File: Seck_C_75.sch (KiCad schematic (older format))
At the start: 122 parts, among them SW1 RESET, U1 ATmega32U4-AU, Y1 16MHz

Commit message: Layout
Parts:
- removed D1, D10, D11, D12, D13, D14, D15, D16, D17, D18, D19, D2, D20, D21, D22, D23, D24, D25, D26, D27, D28, D29, D3, D30, D31, D32, D4, D5, D6, D7, D8, D9: BAV70, Custom_Footprints:SOT-23_Annotated, symbol Diode:BAV70
- removed K_0: KC_ESC, MX_Only:MXOnly-1U-NoLED, symbol Switch:SW_Push
- removed K_013A1: KC_BSPC, MX_Only:MXOnly-1U-NoLED, symbol Switch:SW_Push
- removed K_100: KC_TAB, MX_Only:MXOnly-1.5U-NoLED, symbol Switch:SW_Push
- removed K_101: KC_Q, MX_Only:MXOnly-1U-NoLED, symbol Switch:SW_Push
- removed K_102: KC_W, MX_Only:MXOnly-1U-NoLED, symbol Switch:SW_Push
- removed K_103: KC_E, MX_Only:MXOnly-1U-NoLED, symbol Switch:SW_Push
- removed K_104: KC_R, MX_Only:MXOnly-1U-NoLED, symbol Switch:SW_Push
- removed K_105: KC_T, MX_Only:MXOnly-1U-NoLED, symbol Switch:SW_Push
- removed K_106: KC_Y, MX_Only:MXOnly-1U-NoLED, symbol Switch:SW_Push
- removed K_107: KC_U, MX_Only:MXOnly-1U-NoLED, symbol Switch:SW_Push
- removed K_108: KC_I, MX_Only:MXOnly-1U-NoLED, symbol Switch:SW_Push
- removed K_109: KC_O, MX_Only:MXOnly-1U-NoLED, symbol Switch:SW_Push
- removed K_110: KC_P, MX_Only:MXOnly-1U-NoLED, symbol Switch:SW_Push
- removed K_111: KC_LBRC, MX_Only:MXOnly-1U-NoLED, symbol Switch:SW_Push
- removed K_112: KC_RBRC, MX_Only:MXOnly-1U-NoLED, symbol Switch:SW_Push
- removed K_113: KC_BSLS, MX_Only:MXOnly-1.5U-NoLED, symbol Switch:SW_Push
- removed K_200: KC_CAPS, MX_Only:MXOnly-1.75U-NoLED, symbol Switch:SW_Push
- removed K_200A1: KC_CAPS, MX_Only:MXOnly-1.25U-NoLED, symbol Switch:SW_Push
- removed K_201: KC_A, MX_Only:MXOnly-1U-NoLED, symbol Switch:SW_Push
- removed K_202: KC_S, MX_Only:MXOnly-1U-NoLED, symbol Switch:SW_Push
- removed K_203: KC_D, MX_Only:MXOnly-1U-NoLED, symbol Switch:SW_Push
- removed K_204: KC_F, MX_Only:MXOnly-1U-NoLED, symbol Switch:SW_Push
- removed K_205: KC_G, MX_Only:MXOnly-1U-NoLED, symbol Switch:SW_Push
- removed K_206: KC_H, MX_Only:MXOnly-1U-NoLED, symbol Switch:SW_Push
- removed K_207: KC_J, MX_Only:MXOnly-1U-NoLED, symbol Switch:SW_Push
- removed K_208: KC_K, MX_Only:MXOnly-1U-NoLED, symbol Switch:SW_Push
- removed K_209: KC_L, MX_Only:MXOnly-1U-NoLED, symbol Switch:SW_Push
- removed K_210: KC_SCLN, MX_Only:MXOnly-1U-NoLED, symbol Switch:SW_Push
- removed K_211: KC_QUOT, MX_Only:MXOnly-1U-NoLED, symbol Switch:SW_Push
- removed K_212: KC_ENT, MX_Only:MXOnly-2.25U-NoLED, symbol Switch:SW_Push
- removed K_213: KC_DEL, MX_Only:MXOnly-1U-NoLED, symbol Switch:SW_Push
- removed K_300: KC_LSFT, MX_Only:MXOnly-2.25U-NoLED, symbol Switch:SW_Push
- removed K_301: KC_Z, MX_Only:MXOnly-1U-NoLED, symbol Switch:SW_Push
- removed K_302: KC_X, MX_Only:MXOnly-1U-NoLED, symbol Switch:SW_Push
- removed K_303: KC_C, MX_Only:MXOnly-1U-NoLED, symbol Switch:SW_Push
- removed K_304: KC_V, MX_Only:MXOnly-1U-NoLED, symbol Switch:SW_Push
- removed K_305: KC_B, MX_Only:MXOnly-1U-NoLED, symbol Switch:SW_Push
- removed K_306: KC_N, MX_Only:MXOnly-1U-NoLED, symbol Switch:SW_Push
- removed K_307: KC_M, MX_Only:MXOnly-1U-NoLED, symbol Switch:SW_Push
- removed K_308: KC_COMM, MX_Only:MXOnly-1U-NoLED, symbol Switch:SW_Push
- removed K_309: KC_DOT, MX_Only:MXOnly-1U-NoLED, symbol Switch:SW_Push
- removed K_310: KC_SLSH, MX_Only:MXOnly-1U-NoLED, symbol Switch:SW_Push
- removed K_311: KC_RSFT, MX_Only:MXOnly-2.75U-NoLED, symbol Switch:SW_Push
- removed K_311A1: KC_RSFT, MX_Only:MXOnly-1.75U-NoLED, symbol Switch:SW_Push
- removed K_312, K_410A1: KC_MO(1), MX_Only:MXOnly-1U-NoLED, symbol Switch:SW_Push
- removed K_400: KC_LCTL, MX_Only:MXOnly-1.25U-NoLED, symbol Switch:SW_Push
- removed K_400A1: KC_LCTL, MX_Only:MXOnly-1.5U-NoLED, symbol Switch:SW_Push
- removed K_401: KC_LGUI, MX_Only:MXOnly-1.25U-NoLED, symbol Switch:SW_Push
- removed K_401A1: KC_LGUI, MX_Only:MXOnly-1U-NoLED, symbol Switch:SW_Push
- removed K_402: KC_LALT, MX_Only:MXOnly-1.25U-NoLED, symbol Switch:SW_Push
- removed K_402A1: KC_LALT, MX_Only:MXOnly-1.5U-NoLED, symbol Switch:SW_Push
- removed K_406: KC_SPC, MX_Only:MXOnly-6.25U-ReversedStabilizers-NoLED, symbol Switch:SW_Push
- removed K_406A1: KC_SPC, MX_Only:MXOnly-7U-ReversedStabilizers-NoLED, symbol Switch:SW_Push
- removed K_408: KC_RALT, MX_Only:MXOnly-1.25U-NoLED, symbol Switch:SW_Push
- removed K_409: KC_RGUI, MX_Only:MXOnly-1.25U-NoLED, symbol Switch:SW_Push
- removed K_409A1: KC_RALT, MX_Only:MXOnly-1.5U-NoLED, symbol Switch:SW_Push
- removed K_410: KC_MO(1), MX_Only:MXOnly-1.25U-NoLED, symbol Switch:SW_Push
- removed K_411: KC_RCTL, MX_Only:MXOnly-1.25U-NoLED, symbol Switch:SW_Push
- removed K_411A1: KC_RCTL, MX_Only:MXOnly-1.5U-NoLED, symbol Switch:SW_Push
- added D1, D10, D11, D12, D13, D14, D15, D16, D17, D18, D19, D2, D20, D21, D22, D23, D24, D25, D26, D27, D28, D29, D3, D30, D31, D32, D33, D34, D35, D36, D37, D38, D39, D4, D40, D41, D42, D43, D44, D45, D46, D47, D48, D49, D5, D50, D51, D52, D53, D54, D55, D56, D57, D58, D59, D6, D60, D61, D62, D63, D64, D65, D66, D67, D68, D69, D7, D70, D71, D72, D73, D74, D75, D76, D77, D78, D79, D8, D80, D81, D82, D9: D_Small, Custom_Footprints:D_SOD-123_Annotated, symbol Device:D_Small
- added J1: OLED, Custom_Footprints:SSD1306_OLED, symbol Connector:Conn_01x04_Female
- added K_113A1: KC_BSPC, MX_Only:MXOnly-1U-NoLED, symbol Switch:SW_Push
- added K_14: KC_GRV, MX_Only:MXOnly-1U-NoLED, symbol Switch:SW_Push
- added K_15: KC_1, MX_Only:MXOnly-1U-NoLED, symbol Switch:SW_Push
- added K_16: KC_2, MX_Only:MXOnly-1U-NoLED, symbol Switch:SW_Push
- added K_17: KC_3, MX_Only:MXOnly-1U-NoLED, symbol Switch:SW_Push
- added K_18: KC_4, MX_Only:MXOnly-1U-NoLED, symbol Switch:SW_Push
- added K_19: KC_5, MX_Only:MXOnly-1U-NoLED, symbol Switch:SW_Push
- added K_20: KC_6, MX_Only:MXOnly-1U-NoLED, symbol Switch:SW_Push
- added K_21: KC_7, MX_Only:MXOnly-1U-NoLED, symbol Switch:SW_Push
- added K_22: KC_8, MX_Only:MXOnly-1U-NoLED, symbol Switch:SW_Push
- added K_23: KC_9, MX_Only:MXOnly-1U-NoLED, symbol Switch:SW_Push
- added K_24: KC_0, MX_Only:MXOnly-1U-NoLED, symbol Switch:SW_Push
- added K_25: KC_MINS, MX_Only:MXOnly-1U-NoLED, symbol Switch:SW_Push
- added K_26: KC_EQL, MX_Only:MXOnly-1U-NoLED, symbol Switch:SW_Push
- added K_27: KC_BSPC, MX_Only:MXOnly-2U-NoLED, symbol Switch:SW_Push
- added K_28: KC_DEL, MX_Only:MXOnly-1U-NoLED, symbol Switch:SW_Push
- added K_29: KC_TAB, MX_Only:MXOnly-1.5U-NoLED, symbol Switch:SW_Push
- added K_30: KC_Q, MX_Only:MXOnly-1U-NoLED, symbol Switch:SW_Push
- added K_300A1: KC_CAPS, MX_Only:MXOnly-1.25U-NoLED, symbol Switch:SW_Push
- added K_31: KC_W, MX_Only:MXOnly-1U-NoLED, symbol Switch:SW_Push
- added K_32: KC_E, MX_Only:MXOnly-1U-NoLED, symbol Switch:SW_Push
- added K_33: KC_R, MX_Only:MXOnly-1U-NoLED, symbol Switch:SW_Push
- added K_34: KC_T, MX_Only:MXOnly-1U-NoLED, symbol Switch:SW_Push
- added K_35: KC_Y, MX_Only:MXOnly-1U-NoLED, symbol Switch:SW_Push
- added K_36: KC_U, MX_Only:MXOnly-1U-NoLED, symbol Switch:SW_Push
- added K_37: KC_I, MX_Only:MXOnly-1U-NoLED, symbol Switch:SW_Push
- added K_38: KC_O, MX_Only:MXOnly-1U-NoLED, symbol Switch:SW_Push
- added K_39: KC_P, MX_Only:MXOnly-1U-NoLED, symbol Switch:SW_Push
- added K_40: KC_LBRC, MX_Only:MXOnly-1U-NoLED, symbol Switch:SW_Push
- added K_41: KC_RBRC, MX_Only:MXOnly-1U-NoLED, symbol Switch:SW_Push
- added K_42: KC_BSLS, MX_Only:MXOnly-1.5U-NoLED, symbol Switch:SW_Push
- added K_43: KC_INS, MX_Only:MXOnly-1U-NoLED, symbol Switch:SW_Push
- added K_44: KC_CAPS, MX_Only:MXOnly-1.75U-NoLED, symbol Switch:SW_Push
- added K_45: KC_A, MX_Only:MXOnly-1U-NoLED, symbol Switch:SW_Push
- added K_46: KC_S, MX_Only:MXOnly-1U-NoLED, symbol Switch:SW_Push
- added K_47: KC_D, MX_Only:MXOnly-1U-NoLED, symbol Switch:SW_Push
- added K_48: KC_F, MX_Only:MXOnly-1U-NoLED, symbol Switch:SW_Push
- added K_49: KC_G, MX_Only:MXOnly-1U-NoLED, symbol Switch:SW_Push
- added K_50: KC_H, MX_Only:MXOnly-1U-NoLED, symbol Switch:SW_Push
- added K_508A1: KC_, MX_Only:MXOnly-1.5U-NoLED, symbol Switch:SW_Push
- added K_51: KC_J, MX_Only:MXOnly-1U-NoLED, symbol Switch:SW_Push
- added K_510A1: KC_RCTL, MX_Only:MXOnly-1.5U-NoLED, symbol Switch:SW_Push
- added K_52: KC_K, MX_Only:MXOnly-1U-NoLED, symbol Switch:SW_Push
- added K_53: KC_L, MX_Only:MXOnly-1U-NoLED, symbol Switch:SW_Push
- added K_54: KC_SCLN, MX_Only:MXOnly-1U-NoLED, symbol Switch:SW_Push
- added K_55: KC_QUOT, MX_Only:MXOnly-1U-NoLED, symbol Switch:SW_Push
- added K_56: KC_ENT, MX_Only:MXOnly-2.25U-NoLED, symbol Switch:SW_Push
- added K_57: KC_BSLS, MX_Only:MXOnly-1U-NoLED, symbol Switch:SW_Push
- added K_58: KC_HOME, MX_Only:MXOnly-1U-NoLED, symbol Switch:SW_Push
- added K_59: KC_LSFT, MX_Only:MXOnly-2.25U-NoLED, symbol Switch:SW_Push
- added K_60: KC_Z, MX_Only:MXOnly-1U-NoLED, symbol Switch:SW_Push
- added K_61: KC_X, MX_Only:MXOnly-1U-NoLED, symbol Switch:SW_Push
- added K_62: KC_C, MX_Only:MXOnly-1U-NoLED, symbol Switch:SW_Push
- added K_63: KC_V, MX_Only:MXOnly-1U-NoLED, symbol Switch:SW_Push
- added K_64: KC_B, MX_Only:MXOnly-1U-NoLED, symbol Switch:SW_Push
- added K_65: KC_N, MX_Only:MXOnly-1U-NoLED, symbol Switch:SW_Push
- added K_66: KC_M, MX_Only:MXOnly-1U-NoLED, symbol Switch:SW_Push
- added K_67: KC_COMM, MX_Only:MXOnly-1U-NoLED, symbol Switch:SW_Push
- added K_68: KC_DOT, MX_Only:MXOnly-1U-NoLED, symbol Switch:SW_Push
- added K_69: KC_SLSH, MX_Only:MXOnly-1U-NoLED, symbol Switch:SW_Push
- added K_70: KC_RSFT, MX_Only:MXOnly-1.75U-NoLED, symbol Switch:SW_Push
- added K_71: KC_UP, MX_Only:MXOnly-1U-NoLED, symbol Switch:SW_Push
- added K_72: KC_END, MX_Only:MXOnly-1U-NoLED, symbol Switch:SW_Push
- added K_73: KC_LCTL, MX_Only:MXOnly-1.25U-NoLED, symbol Switch:SW_Push
- added K_74: KC_LGUI, MX_Only:MXOnly-1.25U-NoLED, symbol Switch:SW_Push
- added K_75: KC_LALT, MX_Only:MXOnly-1.25U-NoLED, symbol Switch:SW_Push
- added K_76: KC_SPC, MX_Only:MXOnly-6.25U-ReversedStabilizers-NoLED, symbol Switch:SW_Push
- added K_77: KC_RALT, MX_Only:MXOnly-1U-NoLED, symbol Switch:SW_Push
- added K_78: KC_RGUI, MX_Only:MXOnly-1U-NoLED, symbol Switch:SW_Push
- added K_79: KC_RCTL, MX_Only:MXOnly-1U-NoLED, symbol Switch:SW_Push
- added K_80: KC_LEFT, MX_Only:MXOnly-1U-NoLED, symbol Switch:SW_Push
- added K_81: KC_DOWN, MX_Only:MXOnly-1U-NoLED, symbol Switch:SW_Push
- added K_82: KC_RGHT, MX_Only:MXOnly-1U-NoLED, symbol Switch:SW_Push
- K_1: value KC_1 -> KC_ESC
- K_10: value KC_0 -> KC_F9
- K_11: value KC_MINS -> KC_F10
- K_12: value KC_EQL -> KC_F11
- K_13: value KC_BSPC -> KC_F12; footprint MX_Only:MXOnly-2U-NoLED -> MX_Only:MXOnly-1U-NoLED
- K_2: value KC_2 -> KC_F1
- K_3: value KC_3 -> KC_F2
- K_4: value KC_4 -> KC_F3
- K_5: value KC_5 -> KC_F4
- K_6: value KC_6 -> KC_F5
- K_7: value KC_7 -> KC_F6
- K_8: value KC_8 -> KC_F7
- K_9: value KC_9 -> KC_F8
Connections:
- net +5V: now also J1.2 (Pin_2)
- net GND: now also J1.1 (Pin_1)
- net col0: now also K_1.2, K_14.2, K_29.2, K_300A1.2, K_44.2, K_59.2, K_73.2
- net col1: now also K_2.2, K_15.2, K_30.2, K_45.2, K_60.2, K_74.2; no longer K_1.1
- net col10: now also K_11.2, K_24.2, K_39.2, K_510A1.2, K_54.2, K_69.2, K_79.2; no longer K_10.1
- net col11: now also K_12.2, K_25.2, K_40.2, K_55.2, K_70.2, K_80.2; no longer K_11.1
- net col12: now also K_13.2, K_26.2, K_41.2, K_56.2, K_71.2, K_81.2; no longer K_12.1
- net col13: now also K_113A1.2, K_27.2, K_42.2, K_57.2; no longer K_13.1
- net col2: now also K_3.2, K_16.2, K_31.2, K_46.2, K_61.2, K_75.2; no longer K_2.1
- net col3: now also K_4.2, K_17.2, K_32.2, K_47.2, K_62.2; no longer K_3.1
- net col4: now also K_5.2, K_18.2, K_33.2, K_48.2, K_63.2; no longer K_4.1
- net col5: now also K_6.2, K_19.2, K_34.2, K_49.2, K_64.2; no longer K_5.1
- net col6: now also K_7.2, K_20.2, K_35.2, K_50.2, K_65.2, K_76.2; no longer K_6.1
- net col7: now also K_8.2, K_21.2, K_36.2, K_51.2, K_66.2; no longer K_7.1
- net col8: now also K_9.2, K_22.2, K_37.2, K_508A1.2, K_52.2, K_67.2, K_77.2; no longer K_8.1
- net col9: now also K_10.2, K_23.2, K_38.2, K_53.2, K_68.2, K_78.2; no longer K_9.1
- net row0: now also D1.1 (K), D10.1 (K), D11.1 (K), D12.1 (K), D13.1 (K), D2.1 (K), D3.1 (K), D4.1 (K), D5.1 (K), D6.1 (K), D7.1 (K), D8.1 (K), D9.1 (K)
- net row1: now also D14.1 (K), D15.1 (K), D16.1 (K), D17.1 (K), D18.1 (K), D19.1 (K), D20.1 (K), D21.1 (K), D22.1 (K), D23.1 (K), D24.1 (K), D25.1 (K), D26.1 (K), D27.1 (K), D28.1 (K)
- net row2: now also D29.1 (K), D30.1 (K), D31.1 (K), D32.1 (K), D33.1 (K), D34.1 (K), D35.1 (K), D36.1 (K), D37.1 (K), D38.1 (K), D39.1 (K), D40.1 (K), D41.1 (K), D42.1 (K), D43.1 (K)
- net row3: now also D44.1 (K), D45.1 (K), D46.1 (K), D47.1 (K), D48.1 (K), D49.1 (K), D50.1 (K), D51.1 (K), D52.1 (K), D53.1 (K), D54.1 (K), D55.1 (K), D56.1 (K), D57.1 (K), D58.1 (K)
- net row4: now also D59.1 (K), D60.1 (K), D61.1 (K), D62.1 (K), D63.1 (K), D64.1 (K), D65.1 (K), D66.1 (K), D67.1 (K), D68.1 (K), D69.1 (K), D70.1 (K), D71.1 (K), D72.1 (K)
- net I2C_SCL: now reaches U1.18 (PD0)
- net I2C_SCL: now also J1.3 (Pin_3)
- net I2C_SDA: now reaches U1.19 (PD1)
- net I2C_SDA: now also J1.4 (Pin_4)
- new net: D1.2 (A), K_1.1
- new net: D14.2 (A), K_14.1
- new net: D29.2 (A), K_29.1
- new net: D44.2 (A), K_300A1.1, K_44.1
- new net: D59.2 (A), K_59.1
- new net: D73.2 (A), K_73.1
- new net: D2.2 (A), K_2.1
- new net: D15.2 (A), K_15.1
- new net: D30.2 (A), K_30.1
- new net: D45.2 (A), K_45.1
- new net: D60.2 (A), K_60.1
- new net: D74.2 (A), K_74.1
- new net: D3.2 (A), K_3.1
- new net: D16.2 (A), K_16.1
- new net: D31.2 (A), K_31.1
- new net: D46.2 (A), K_46.1
- new net: D61.2 (A), K_61.1
- new net: D75.2 (A), K_75.1
- new net: D4.2 (A), K_4.1
- new net: D17.2 (A), K_17.1
- new net: D32.2 (A), K_32.1
- new net: D47.2 (A), K_47.1
- new net: D62.2 (A), K_62.1
- new net: D5.2 (A), K_5.1
- new net: D18.2 (A), K_18.1
- new net: D33.2 (A), K_33.1
- new net: D48.2 (A), K_48.1
- new net: D63.2 (A), K_63.1
- new net: D6.2 (A), K_6.1
- new net: D19.2 (A), K_19.1
- new net: D34.2 (A), K_34.1
- new net: D49.2 (A), K_49.1
- new net: D64.2 (A), K_64.1
- new net: D7.2 (A), K_7.1
- new net: D20.2 (A), K_20.1
- new net: D35.2 (A), K_35.1
- new net: D50.2 (A), K_50.1
- new net: D65.2 (A), K_65.1
- new net: D76.2 (A), K_76.1
- new net: D77.2 (A), K_508A1.1, K_77.1
- new net: D8.2 (A), K_8.1
- new net: D21.2 (A), K_21.1
- new net: D36.2 (A), K_36.1
- new net: D51.2 (A), K_51.1
- new net: D66.2 (A), K_66.1
- new net: D9.2 (A), K_9.1
- new net: D22.2 (A), K_22.1
- new net: D37.2 (A), K_37.1
- new net: D52.2 (A), K_52.1
- new net: D67.2 (A), K_67.1
- new net: D10.2 (A), K_10.1
- new net: D23.2 (A), K_23.1
- new net: D38.2 (A), K_38.1
- new net: D53.2 (A), K_53.1
- new net: D68.2 (A), K_68.1
- new net: D78.2 (A), K_78.1
- new net: D11.2 (A), K_11.1
- new net: D24.2 (A), K_24.1
- new net: D39.2 (A), K_39.1
- new net: D54.2 (A), K_54.1
- new net: D69.2 (A), K_69.1
- new net: D79.2 (A), K_510A1.1, K_79.1
- new net: D12.2 (A), K_12.1
- new net: D25.2 (A), K_25.1
- new net: D40.2 (A), K_40.1
- new net: D55.2 (A), K_55.1
- new net: D70.2 (A), K_70.1
- new net: D80.2 (A), K_80.1
- new net: D13.2 (A), K_13.1
- new net: D26.2 (A), K_26.1
- new net: D41.2 (A), K_41.1
- new net: D56.2 (A), K_56.1
- new net: D71.2 (A), K_71.1
- new net: D81.2 (A), K_81.1
- new net: D27.2 (A), K_113A1.1, K_27.1
- new net: D42.2 (A), K_42.1
- new net: D57.2 (A), K_57.1
- new net: D28.2 (A), K_28.1
- new net: D43.2 (A), K_43.1
- new net: D58.2 (A), K_58.1
- new net: D72.2 (A), K_72.1
- new net: D82.2 (A), K_82.1
- new net col14: K_28.2, K_43.2, K_58.2, K_72.2, K_82.2
- new net row5: D73.1 (K), D74.1 (K), D75.1 (K), D76.1 (K), D77.1 (K), D78.1 (K), D79.1 (K), D80.1 (K), D81.1 (K), D82.1 (K)
- no-connect marks 4 -> 3
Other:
- moved on the sheet: C1, C2, C3, C4, C5, ESD1, F1, R1, R2, R3, R4, R5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

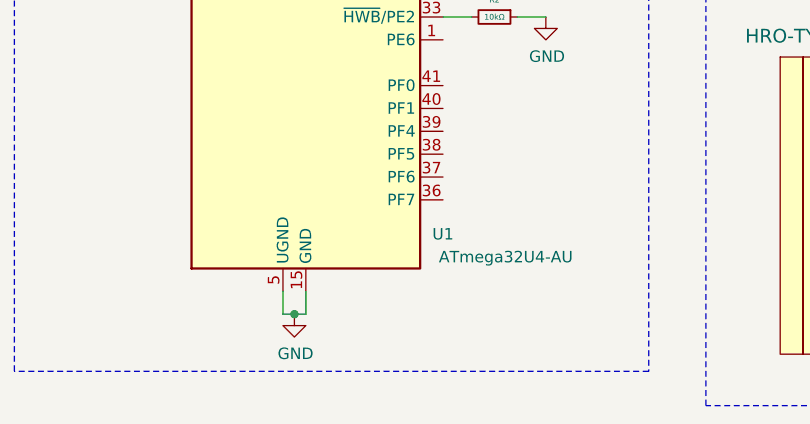
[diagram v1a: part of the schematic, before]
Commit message: Diodes
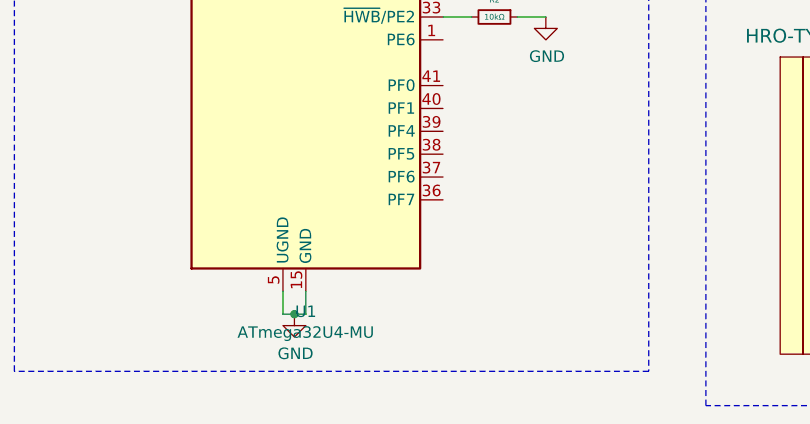
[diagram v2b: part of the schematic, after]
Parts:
- removed U1: ATmega32U4-AU, Custom_Footprints:ATMEGA32U4_Annotated, symbol MCU_Microchip_ATmega:ATmega32U4-AU
- added U1: ATmega32U4-MU, Package_DFN_QFN:QFN-44-1EP_7x7mm_P0.5mm_EP5.2x5.2mm, symbol MCU_Microchip_ATmega:ATmega32U4-MU
- D1, D10, D11, D12, D13, D14, D15, D16, D17, D18, D19, D2, D20, D21, D22, D23, D24, D25, D26, D27, D28, D29, D3, D30, D31, D32, D33, D34, D35, D36, D37, D38, D39, D4, D40, D41, D42, D43, D44, D45, D46, D47, D48, D49, D5, D50, D51, D52, D53, D54, D55, D56, D57, D58, D59, D6, D60, D61, D62, D63, D64, D65, D66, D67, D68, D69, D7, D70, D71, D72, D73, D74, D75, D76, D77, D78, D79, D8, D80, D81, D82, D9: footprint Custom_Footprints:D_SOD-123_Annotated -> Diode_SMD:D_0603_1608Metric_Pad1.05x0.95mm_HandSolder
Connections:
- net +5V: now also U1.14 (VCC), U1.2 (UVCC), U1.24 (AVCC), U1.34 (VCC), U1.44 (AVCC), U1.7 (VBUS)
- net DA+: now also U1.4 (D+)
- net DA-: now also U1.3 (D-)
- net GND: now also U1.15 (GND), U1.23 (GND), U1.35 (GND), U1.43 (GND), U1.45 (GND), U1.5 (UGND)
- net I2C_SCL: now also U1.18 (PD0)
- net I2C_SDA: now also U1.19 (PD1)
- net at R1.2, SW1.2: now also U1.13 (~RESET)
- net at Y1.3: now also U1.16 (XTAL2)
- net at Y1.1: now also U1.17 (XTAL1)
- net at R2.2: now also U1.33 (~HWB~/PE2)
- net at C5.1: now also U1.6 (UCAP)

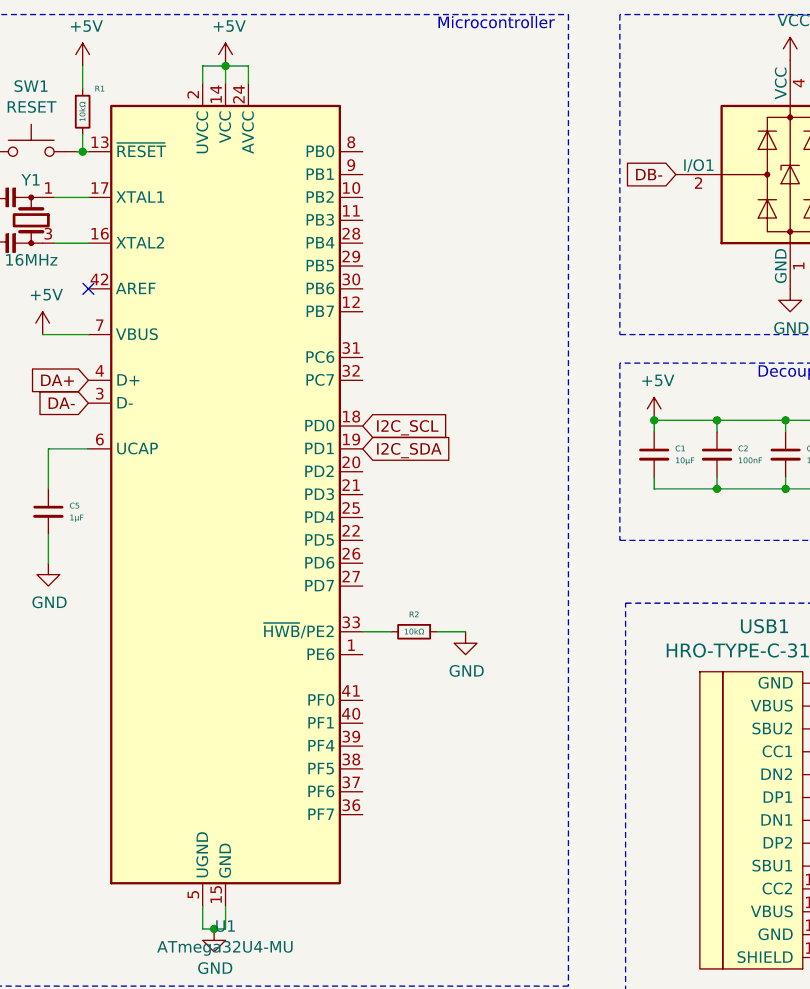
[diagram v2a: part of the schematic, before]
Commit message: Finish
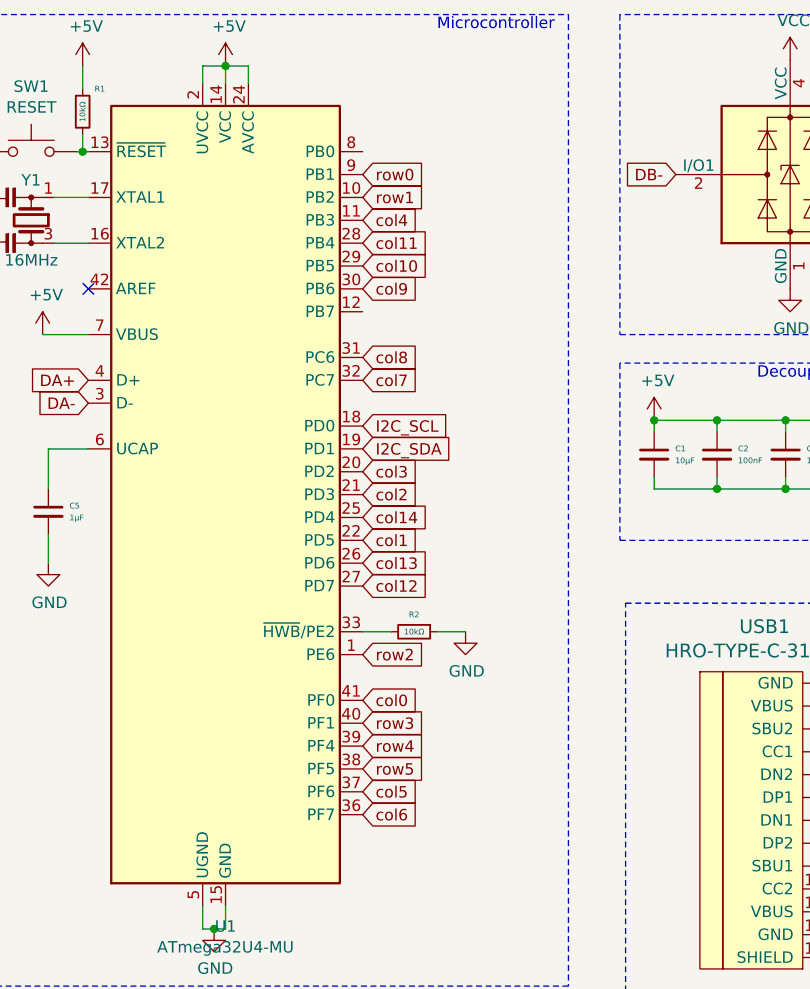
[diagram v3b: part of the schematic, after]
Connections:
- net col0: now also U1.41 (PF0)
- net col1: now also U1.22 (PD5)
- net col10: now also U1.29 (PB5)
- net col11: now also U1.28 (PB4)
- net col12: now also U1.27 (PD7)
- net col13: now also U1.26 (PD6)
- net col14: now also U1.25 (PD4)
- net col2: now also U1.21 (PD3)
- net col3: now also U1.20 (PD2)
- net col4: now also U1.11 (PB3)
- net col5: now also U1.37 (PF6)
- net col6: now also U1.36 (PF7)
- net col7: now also U1.32 (PC7)
- net col8: now also U1.31 (PC6)
- net col9: now also U1.30 (PB6)
- net row0: now also U1.9 (PB1)
- net row1: now also U1.10 (PB2)
- net row2: now also U1.1 (PE6)
- net row3: now also U1.40 (PF1)
- net row4: now also U1.39 (PF4)
- net row5: now also U1.38 (PF5)
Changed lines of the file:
@@
 	1    0    0    -1
 $EndComp
+Text GLabel 12650 4200 2    50   Input ~ 0
+col0
+Text GLabel 12650 4000 2    50   Input ~ 0
+row2
+Text GLabel 12650 4300 2    50   Input ~ 0
+row3
+Text GLabel 12650 4400 2    50   Input ~ 0
+row4
+Text GLabel 12650 4500 2    50   Input ~ 0
+row5
+Text GLabel 12650 3500 2    50   Input ~ 0
+col1
+Text GLabel 12650 3300 2    50   Input ~ 0
+col2
+Text GLabel 12650 3200 2    50   Input ~ 0
+col3
+Text GLabel 12650 3400 2    50   Input ~ 0
+col14
+Text GLabel 12650 3600 2    50   Input ~ 0
+col13
+Text GLabel 12650 3700 2    50   Input ~ 0
+col12
+Text GLabel 12650 2200 2    50   Input ~ 0
+col11
+Text GLabel 12650 2300 2    50   Input ~ 0
+col10
+Text GLabel 12650 2400 2    50   Input ~ 0
+col9
+Text GLabel 12650 2700 2    50   Input ~ 0
+col8
+Text GLabel 12650 2800 2    50   Input ~ 0
+col7
+Text GLabel 12650 4700 2    50   Input ~ 0
+col6
+Text GLabel 12650 4600 2    50   Input ~ 0
+col5
+Text GLabel 12650 2100 2    50   Input ~ 0
+col4
+Text GLabel 12650 1900 2    50   Input ~ 0
+row0
+Text GLabel 12650 2000 2    50   Input ~ 0
+row1
 $EndSCHEMATC

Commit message: Make Gerbers + add Art
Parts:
- C1: LCSC (none) -> C19702
- C2, C3, C4: LCSC (none) -> C14663
- C5: LCSC (none) -> C15849
- D1, D10, D11, D12, D13, D14, D15, D16, D17, D18, D19, D2, D20, D21, D22, D23, D24, D25, D26, D27, D28, D29, D3, D30, D31, D32, D33, D34, D35, D36, D37, D38, D39, D4, D40, D41, D42, D43, D44, D45, D46, D47, D48, D49, D5, D50, D51, D52, D53, D54, D55, D56, D57, D58, D59, D6, D60, D61, D62, D63, D64, D65, D66, D67, D68, D69, D7, D70, D71, D72, D73, D74, D75, D76, D77, D78, D79, D8, D80, D81, D82, D9: LCSC (none) -> C109002
- R1, R2: LCSC (none) -> C25804
- R3, R4: LCSC (none) -> C23345
- R5, R6: LCSC (none) -> C23186
- U1: LCSC (none) -> C45874
